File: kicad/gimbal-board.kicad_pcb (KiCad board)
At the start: 2 copper layers, 79 x 45 mm, 34 parts, among them IC1 ATMEGA328P-A, P1 ICSP_CONN, P2 BAT_CONN, P3 MOTOR_CONN, P4 IMU_CONN, P5 FTDI_CONN, P6 3V3_CONN, SW1 SW_PUSH, SW2 SW_PUSH, U1 DRV10975, Y1 Resonator

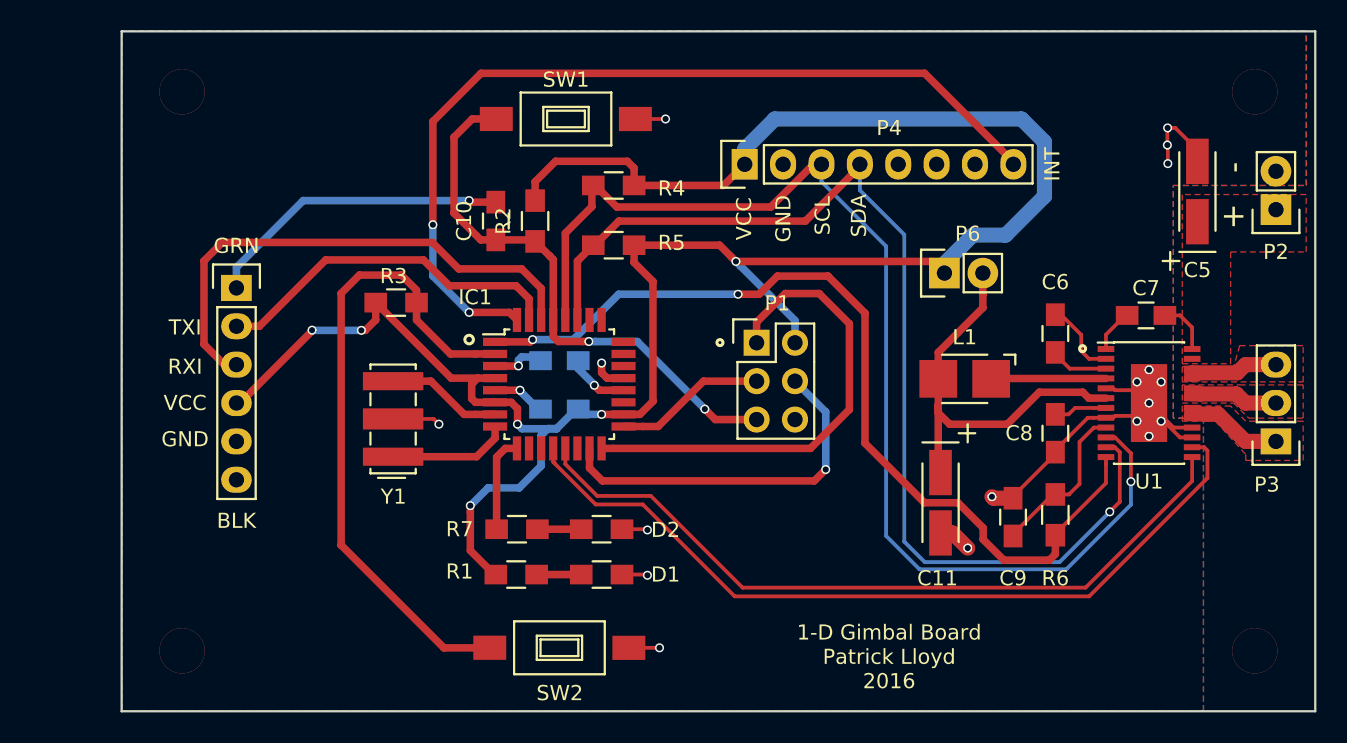
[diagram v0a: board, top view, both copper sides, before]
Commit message: Remade Rev 01 layout and sent to fab
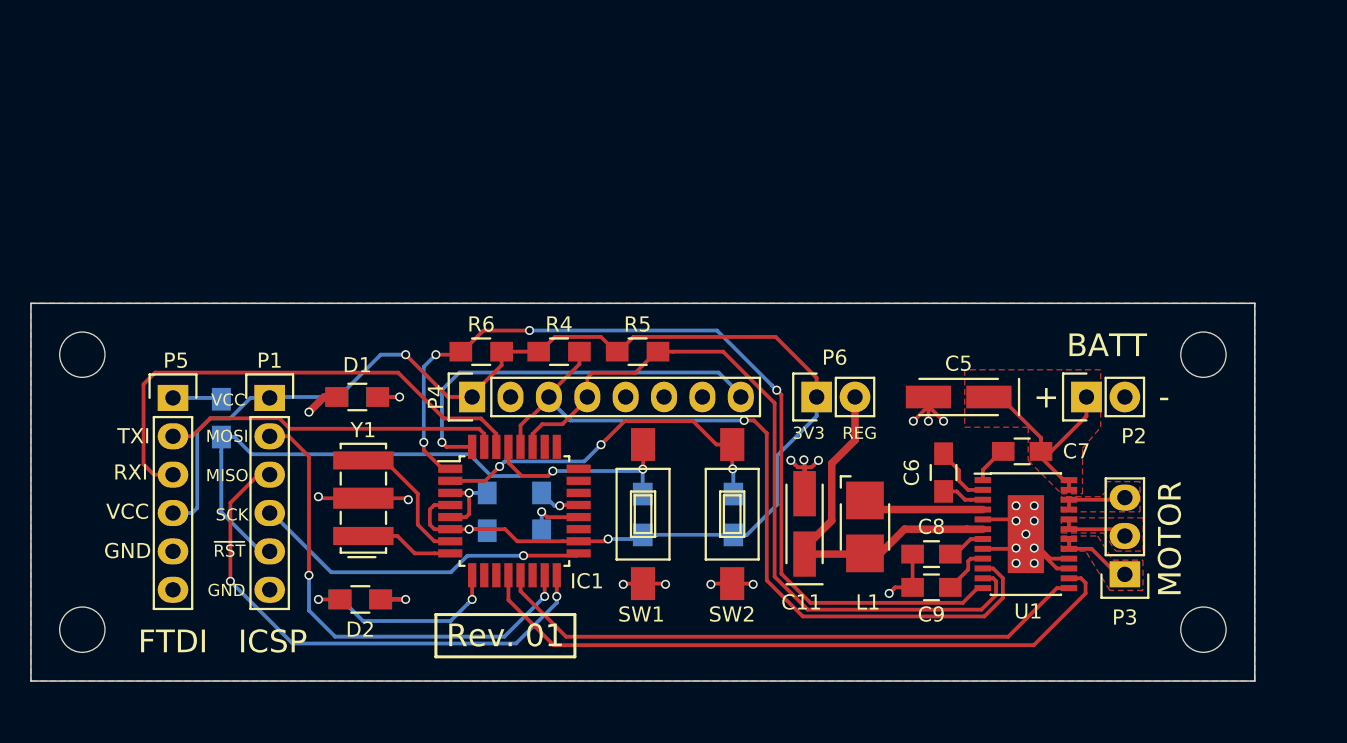
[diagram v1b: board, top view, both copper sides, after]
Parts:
- C10, R1, R2, R3, R7: moved to B.Cu
- C11, C5: footprint Capacitors_Tantalum_SMD:TantalC_SizeA_EIA-3216_HandSoldering -> gimbal-board:TantalC_SizeA_EIA-3216_HandSoldering
- P1: value ICSP_CONN -> ICSP; footprint Pin_Headers:Pin_Header_Straight_2x03 -> Pin_Headers:Pin_Header_Straight_1x06
- P2: value BAT_CONN -> BATT
- P3: value MOTOR_CONN -> MOTOR
- P4: value IMU_CONN -> IMU
- P5: value FTDI_CONN -> FTDI
- moved H3 79.5 mm to (97.4, 46.4)
- moved H1 77.6 mm to (97.4, 64.6)
- moved H4 69.8 mm to (171.6, 46.4)
- moved H2 67.6 mm to (171.6, 64.6)
- moved R6 39.5 mm to (123.8, 46.2), turned to 180 degrees
- moved P1 32.4 mm to (109.8, 49.3)
- moved SW1 26.6 mm to (134.5, 56.9), turned to 270 degrees
- moved R3 26.4 mm to (140.5, 57.0), turned to 270 degrees
- moved P4 23.7 mm to (123.2, 49.2)
- moved C10 22.4 mm to (106.6, 50.6)
- moved C5 20.8 mm to (155.4, 49.2), turned to 180 degrees
- moved R2 20.7 mm to (134.5, 57.0), turned to 270 degrees
- moved D1 20.0 mm to (115.6, 49.2), turned to 0 degrees
- moved P2 17.6 mm to (163.9, 49.2), turned to 90 degrees
- moved D2 16.6 mm to (115.8, 62.6), turned to 0 degrees
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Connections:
- P1 pad 1: /ICSP_MISO -> +3V3
- P1 pad 2: +3V3 -> /ICSP_MOSI
- P1 pad 3: /ICSP_SCK -> /ICSP_MISO
- P1 pad 4: /ICSP_MOSI -> /ICSP_SCK
- R6 pad 1: /V3P3 -> +3V3
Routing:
- net +3V3: track 144.7 -> 92.9 mm, vias 6 -> 3
- net /IMU_INT: track 59.3 -> 26.6 mm, vias 2 -> 1
- net /SCL: track 77.6 -> 53.3 mm
- net /SDA: track 72.3 -> 50.7 mm, vias 1 -> 0
- net Net-(IC1-Pad2): track 43.4 -> 24.3 mm, vias 0 -> 3
- net /USART_DTR: track 20.4 -> 3.24 mm, vias 1 -> 0
- net /ICSP_SCK: track 10.1 -> 22.6 mm, vias 0 -> 1
- net +BATT: track 3.56 -> 14.2 mm
- net /M_SPEED: track 50.4 -> 39.9 mm
- net /M_DIR: track 54.1 -> 44.4 mm
- net /RESET: track 37.1 -> 46.2 mm
- net /ICSP_MOSI: track 24.3 -> 32.2 mm, vias 1 -> 2
- net /V3P3: track 10.8 -> 3.26 mm
- net Net-(IC1-Pad9): track 6.36 -> 11.5 mm, vias 0 -> 1
- net /REG_OUT: track 27.4 -> 24.3 mm
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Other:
- board size 79 x 45 mm -> 81 x 25 mm
- rule pad_to_mask_clearance: 0.2 -> 0
- board text added: "1D BLDC Gimbal Patrick Lloyd 2016"
- board text added: "3V3"
- board text added: "BATT"
- board text added: "FTDI"
- board text added: "GY-521 Breakout"
- board text added: "ICSP"
- board text added: "MISO"
- board text added: "MOSI"
- board text added: "MOTOR"
- board text added: "REG"
- board text added: "Rev. 01"
- board text added: "SCK"
- board text added: "~RST"
- board text removed: "1-D Gimbal Board Patrick Lloyd 2016"
- board text removed: "BLK"
- board text removed: "GRN"
- board text removed: "INT"
- board text removed: "SCL"
- board text removed: "SDA"
